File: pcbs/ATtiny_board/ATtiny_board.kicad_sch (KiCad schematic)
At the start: 1 part, among them U1 ATtiny85V-10P

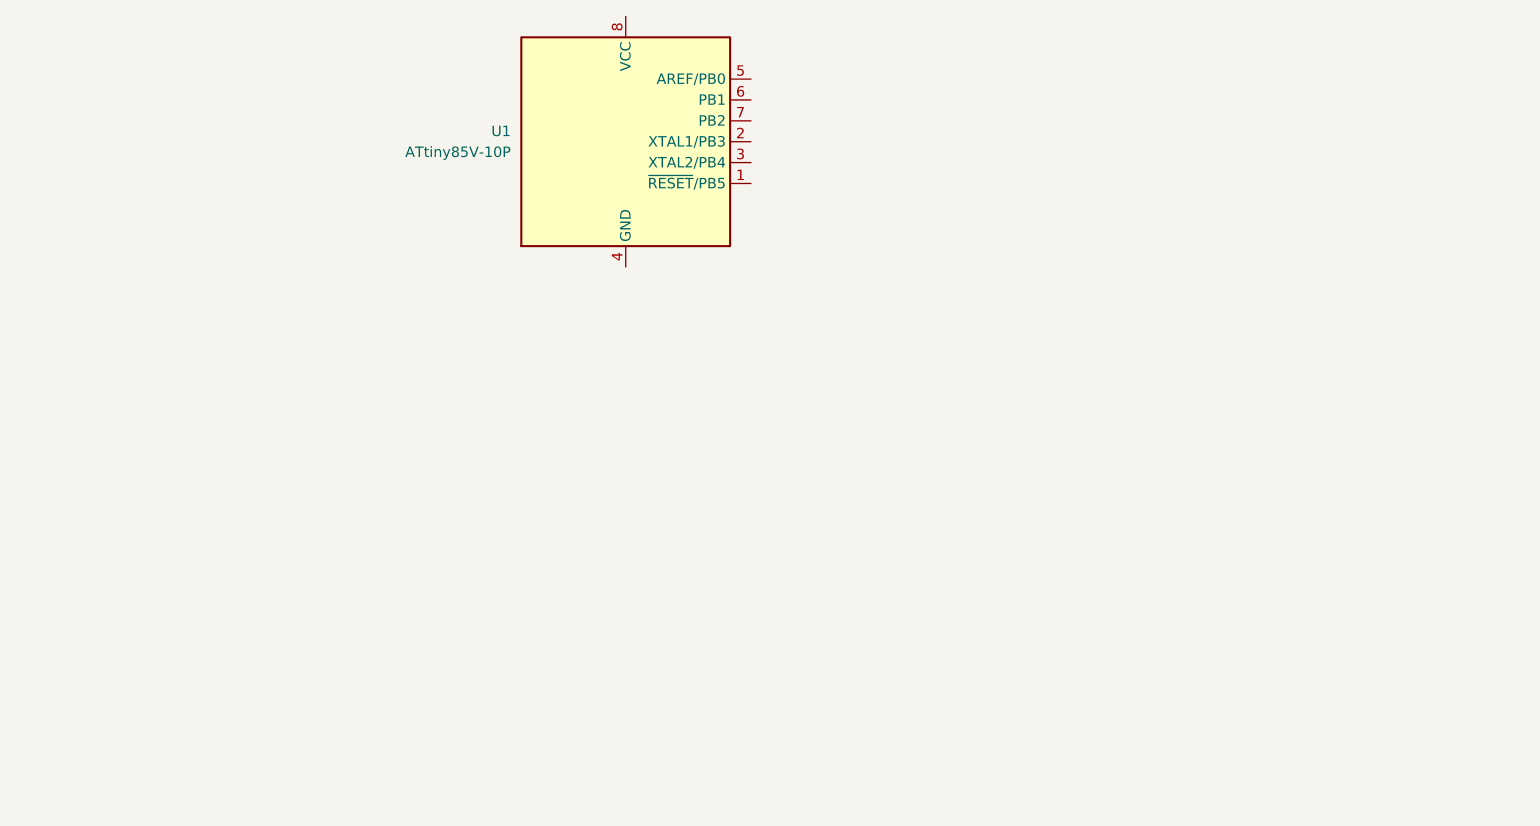
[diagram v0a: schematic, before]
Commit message: Designing PCB
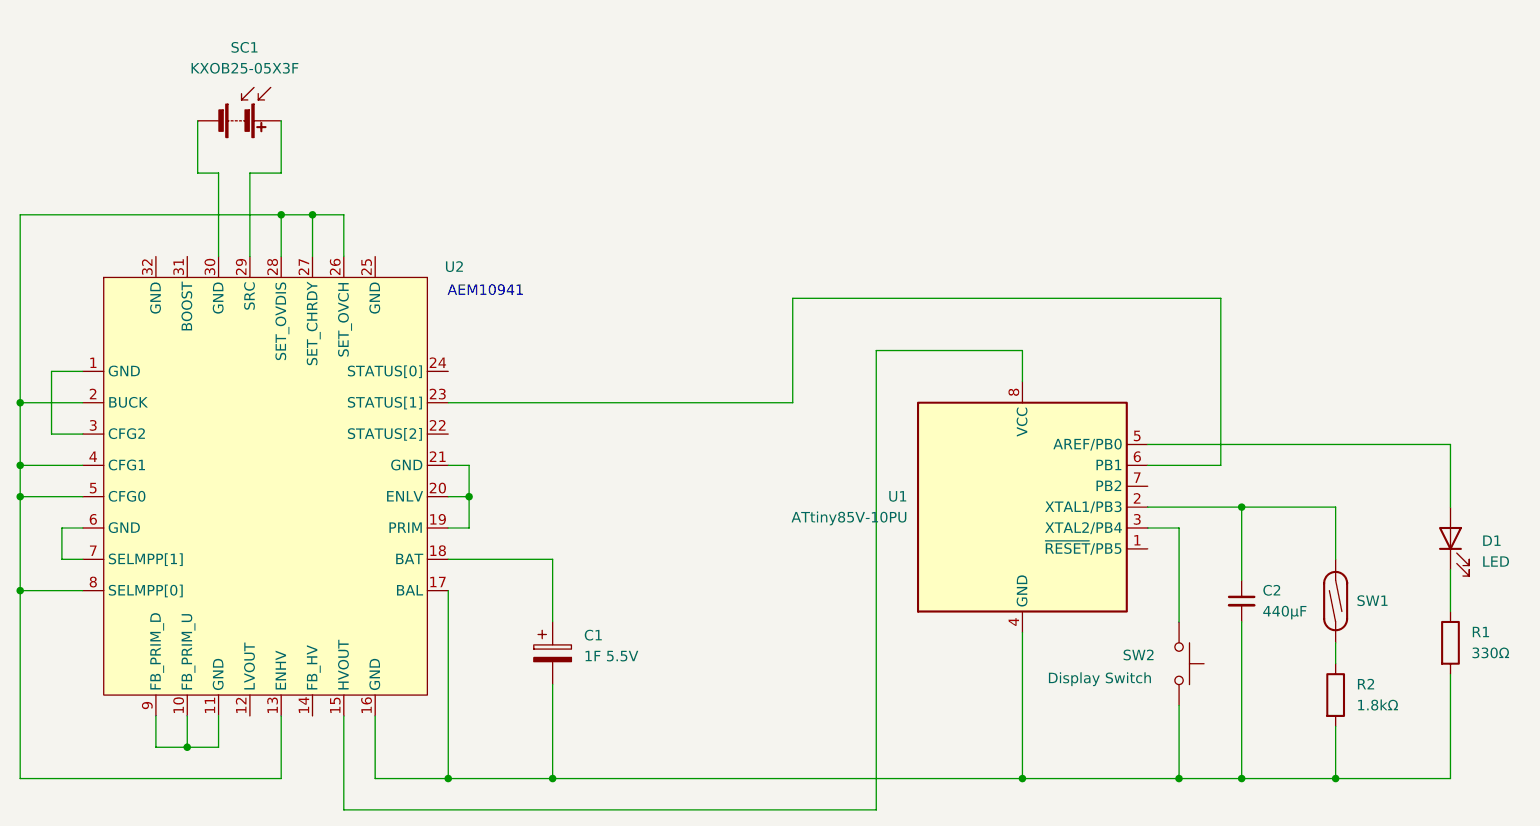
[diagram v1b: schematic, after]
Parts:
- added C1: 1F 5.5V, symbol Device:C_Polarized
- added C2: 440μF, symbol Device:C_Small
- added D1: LED, symbol Device:LED
- added R1: 330Ω, symbol Device:R
- added R2: 1.8kΩ, symbol Device:R
- added SC1: KXOB25-05X3F, symbol Device:Solar_Cells
- added SW1: (no value), symbol Switch:SW_Reed
- added SW2: Display Switch, symbol Switch:SW_Push
- added U2: (no value), energy_harvest:AEM10941_board, symbol new_ivo_lib:AEM10941_board
- U1: value ATtiny85V-10P -> ATtiny85V-10PU
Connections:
- net at U1.2 (XTAL1/PB3): now also C2.1, SW1.2
- net at U1.3 (XTAL2/PB4): now also SW2.1
- net at U1.4 (GND): now also C1.2, C2.2, R1.2, R2.2, SW2.2, U2.16 (GND), U2.17 (BAL)
- net at U1.5 (AREF/PB0): now also D1.2 (A)
- net at U1.6 (PB1): now also U2.23 (STATUS[1])
- net at U1.8 (VCC): now also U2.15 (HVOUT)
- new net: R2.1, SW1.1
- new net: D1.1 (K), R1.1
- new net: U2.1 (GND), U2.3 (CFG2)
- new net: U2.10 (FB_PRIM_U), U2.11 (GND), U2.9 (FB_PRIM_D)
- new net: U2.13 (ENHV), U2.2 (BUCK), U2.26 (SET_OVCH), U2.27 (SET_CHRDY), U2.28 (SET_OVDIS), U2.4 (CFG1), U2.5 (CFG0), U2.8 (SELMPP[0])
- new net: C1.1, U2.18 (BAT)
- new net: U2.19 (PRIM), U2.20 (ENLV), U2.21 (GND)
- new net: SC1.1 (+), U2.29 (SRC)
- new net: SC1.2 (-), U2.30 (GND)
- new net: U2.6 (GND), U2.7 (SELMPP[1])
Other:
- note added: "AEM10941"
- moved on the sheet: U1
